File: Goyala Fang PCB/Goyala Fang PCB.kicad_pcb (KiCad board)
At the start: 2 copper layers, 45 x 20 mm, 8 parts, among them J2 Conn_01x06, U3 L298N, U5 MPU-6050, U6 INA219AxD

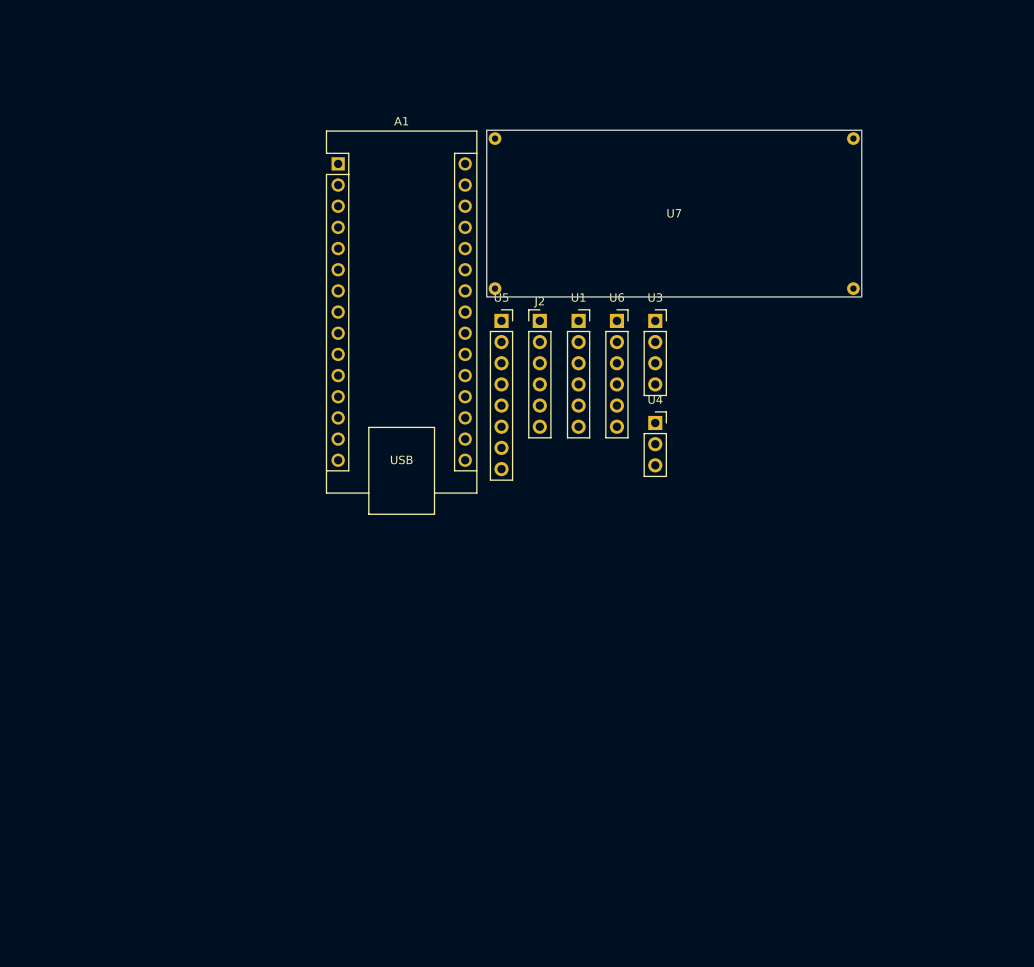
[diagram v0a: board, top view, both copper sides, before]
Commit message: [Feat] Added App
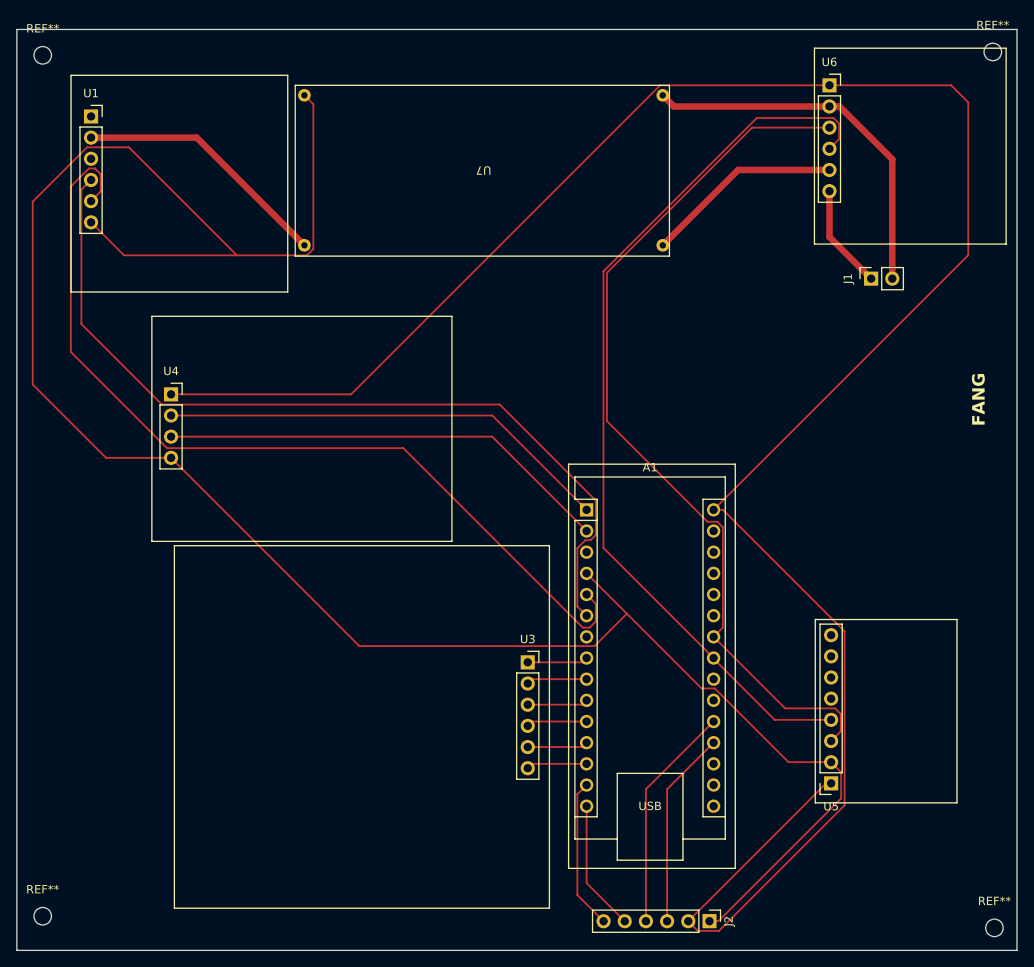
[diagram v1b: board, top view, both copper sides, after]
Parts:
- added J1: Input Battery, Connector_PinSocket_2.54mm:PinSocket_1x02_P2.54mm_Vertical, F.Cu at (180.5, 83.9)
- added REF**: MountingHole_2.1mm, MountingHole:MountingHole_2.1mm, F.Cu at (81.1, 160.4)
- added REF**: MountingHole_2.1mm, MountingHole:MountingHole_2.1mm, F.Cu at (81.1, 57.1)
- added REF**: MountingHole_2.1mm, MountingHole:MountingHole_2.1mm, F.Cu at (195.1, 56.7)
- added REF**: MountingHole_2.1mm, MountingHole:MountingHole_2.1mm, F.Cu at (195.3, 161.8)
- U3: footprint Connector_PinSocket_2.54mm:PinSocket_1x04_P2.54mm_Vertical -> Connector_PinSocket_2.54mm:PinSocket_1x06_P2.54mm_Vertical
- U4: footprint Connector_PinSocket_2.54mm:PinSocket_1x03_P2.54mm_Vertical -> Connector_PinSocket_2.54mm:PinSocket_1x04_P2.54mm_Vertical
- moved J2 74.8 mm to (161.1, 161.0), turned to -90 degrees
- moved U5 68.1 mm to (175.7, 144.5), turned to 180 degrees
- moved U1 63.4 mm to (86.9, 64.4)
- moved U4 58.2 mm to (96.5, 97.8)
- moved A1 51.1 mm to (146.4, 111.6)
- moved U3 43.7 mm to (139.3, 129.9)
- moved U6 38.1 mm to (175.5, 60.7)
- moved U7 23.7 mm to (134.0, 70.4), turned to 180 degrees
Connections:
- A1 pad 11: ena -> in2
- A1 pad 12: in2 -> in1
- A1 pad 13: in1 -> ena
- A1 pad 7: in1 -> unconnected-(A1-D4-Pad7)
- J2 pad 3: Net-(A1-D12) -> Net-(A1-A0)
- J2 pad 5: Net-(A1-A0) -> Net-(A1-D12)
- U1 pad 3: GND -> unconnected-(U1-RST-Pad3)
- U1 pad 6: unconnected-(U1-RST-Pad6) -> GND
- U4 pad 2: GND -> Net-(A1-D1/TX)
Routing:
- net GND: track 0.00 -> 298.4 mm
- net +5V: track 0.00 -> 265.5 mm
- net sda: track 0.00 -> 109.7 mm
- net Net-(A1-D2): track 0.00 -> 109.0 mm
- net scl: track 0.00 -> 107.3 mm
- net Net-(A1-D3): track 0.00 -> 103.8 mm
- net Net-(A1-D1/TX): track 0.00 -> 54.5 mm
- net Net-(A1-D0/RX): track 0.00 -> 54.5 mm
- net +3.3V: track 0.00 -> 31.0 mm
- net Net-(A1-A1): track 0.00 -> 27.3 mm
- net Net-(U3-Vs): track 0.00 -> 23.7 mm
- net Net-(A1-A0): track 0.00 -> 23.7 mm
- net Net-(A1-D11): track 0.00 -> 18.1 mm
- net Net-(A1-D12): track 0.00 -> 15.7 mm
- net Net-(J1-Pin_1): track 0.00 -> 12.6 mm
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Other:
- board size 45 x 20 mm -> 120 x 110.5 mm
- board text added: "FANG"
